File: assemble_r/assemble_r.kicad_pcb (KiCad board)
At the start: 2 copper layers, 128.5 x 92.1 mm, 45 parts, among them J23 Conn_01x02_Pin, SW23 SW_Push, SW24 SW_Push, SW25 SW_Push, SW26 SW_Push, SW27 SW_Push, SW28 SW_Push, SW29 SW_Push, SW30 SW_Push, SW31 SW_Push, SW32 SW_Push, SW33 SW_Push, SW34 SW_Push, SW35 SW_Push, SW36 SW_Push, SW37 SW_Push, SW38 SW_Push, SW39 SW_Push, SW40 SW_Push, SW41 SW_Push, SW42 SW_Push, SW43 SW_Push, SW44 SW_Push, U23 Micon_BLEMicroPro

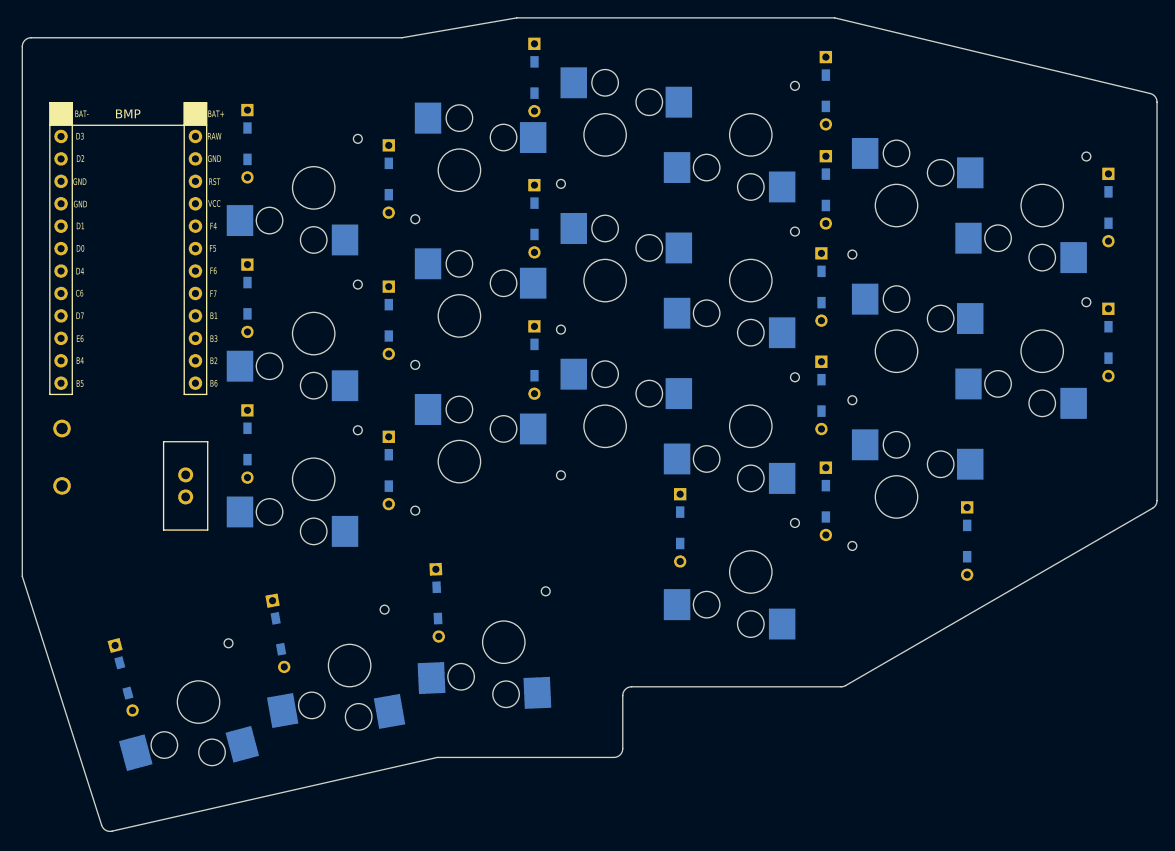
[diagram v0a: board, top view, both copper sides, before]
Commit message: fix: re-change layout
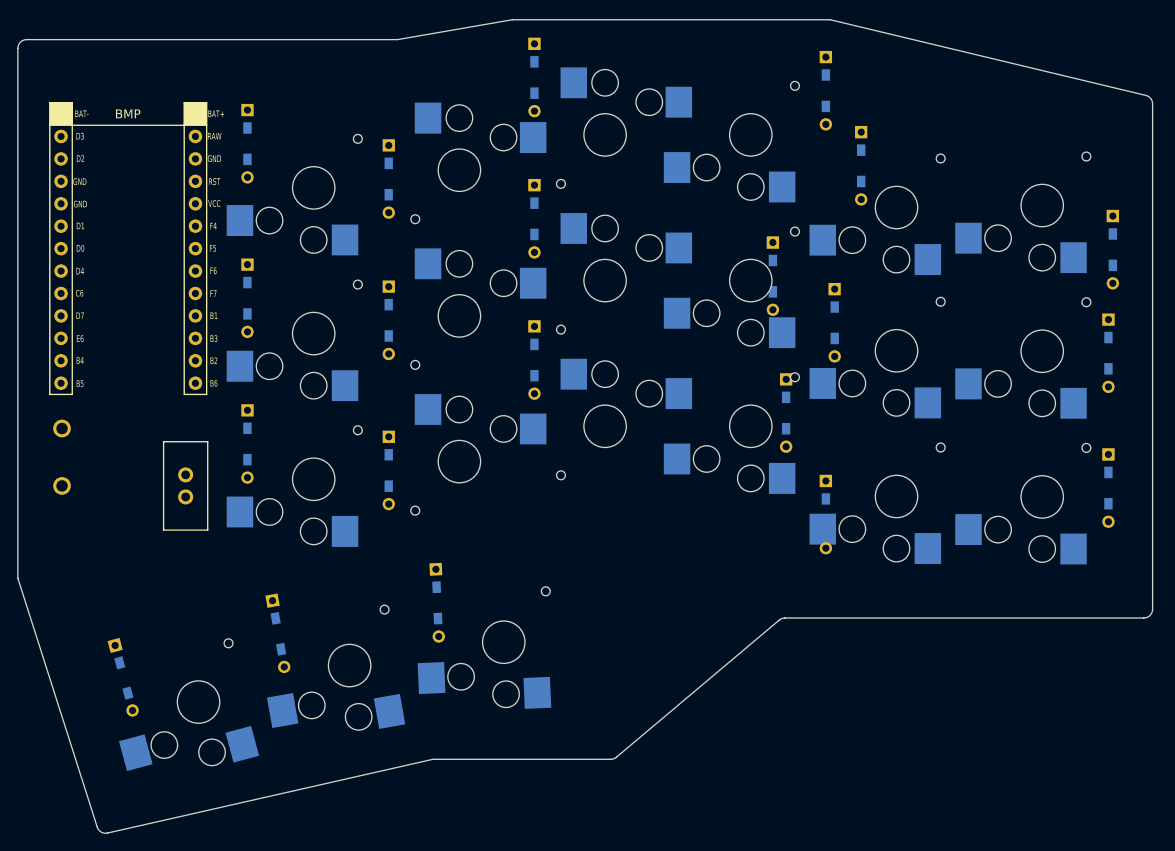
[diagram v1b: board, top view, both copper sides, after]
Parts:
- moved D38 45.8 mm to (133.0, 46.5)
- moved SW38 44.5 mm to (137.0, 51.2)
- moved D41 36.9 mm to (161.5, 56.0)
- moved SW41 36.9 mm to (153.5, 51.0), turned to 0 degrees
- moved D43 16.5 mm to (161.0, 83.0)
- moved SW42 16.5 mm to (153.5, 67.5)
- moved SW43 16.5 mm to (153.5, 84.0)
- moved D42 16.5 mm to (161.0, 67.7)
- moved SW39 16.5 mm to (137.0, 67.5), turned to 0 degrees
- moved SW40 16.5 mm to (137.0, 84.0), turned to 0 degrees
- moved D39 15.1 mm to (130.0, 64.3)
- moved D40 13.5 mm to (129.0, 86.0)
- moved D37 11.0 mm to (124.5, 74.5)
- moved D36 5.63 mm to (123.0, 59.0)
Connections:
- D38 pad 1: Row3 -> Row2
- SW38 pad 1: Col3 -> Col5
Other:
- outline, holes or cut-outs redrawn
